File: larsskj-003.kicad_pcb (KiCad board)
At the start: 2 copper layers, 47.6 x 39 mm, 14 parts, among them J1 IDC connector, J2 Conn_02x01, J3 Conn_02x01, J4 Conn_02x01, J5 Conn_02x01, J6 Conn_02x01, J7 Conn_02x01, J8 Conn_02x01, J9 Conn_02x01

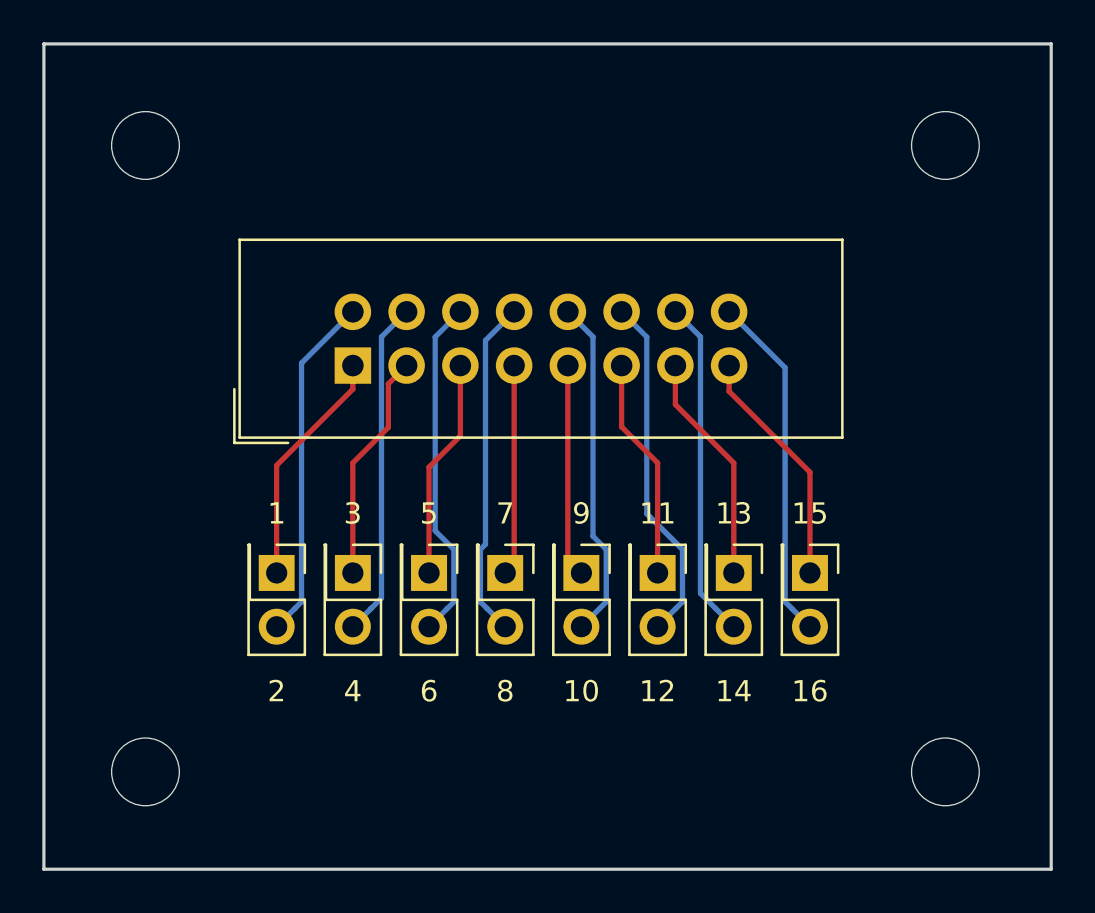
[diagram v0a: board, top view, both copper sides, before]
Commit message: Improved PCB layout
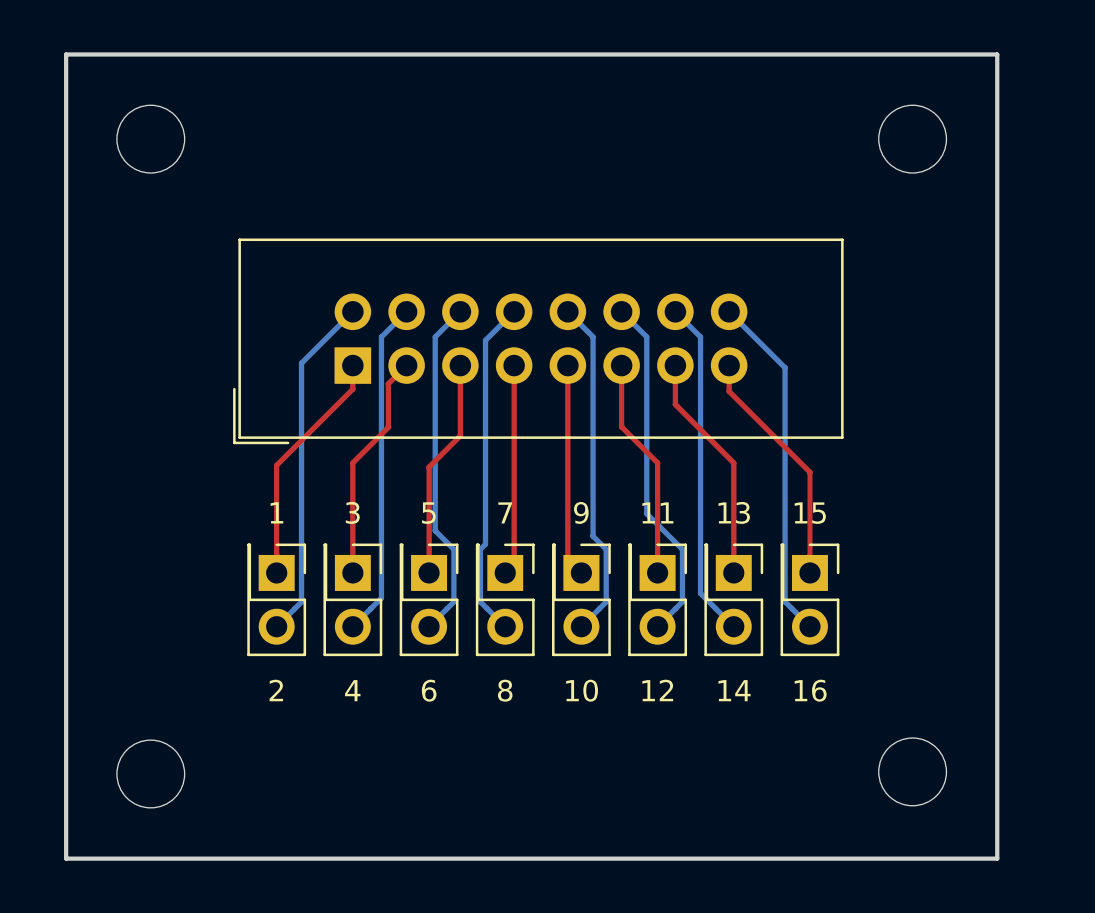
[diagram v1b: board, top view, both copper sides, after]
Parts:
- moved REF** 1.58 mm to (160.7, 80.3)
- moved REF** 1.55 mm to (160.7, 110.2)
- moved REF** 1.45 mm to (152.7, 95.8)
- moved REF** 0.39 mm to (124.7, 80.3)
- moved REF** 0.27 mm to (124.7, 110.3)
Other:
- board size 47.6 x 39 mm -> 44 x 38 mm
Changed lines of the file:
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@@
-(kicad_pcb (version 20171130) (host pcbnew "(5.0.1)-3")
+(kicad_pcb (version 20171130) (host pcbnew 5.0.2-bee76a0~70~ubuntu18.04.1)
   (general
     (thickness 1.6)
@@
     (solder_mask_min_width 0.25)
     (aux_axis_origin 0 0)
+    (grid_origin 120.65 114.3)
     (visible_elements 7FFFFFFF)
     (pcbplotparams
@@
   )
   (module MountingHole:MountingHole_3.2mm_M3 (layer F.Cu)
-    (at 162.2 110.2)
+    (at 160.65 110.2)
     (descr "Mounting Hole 3.2mm, no annular, M3")
     (tags "mounting hole 3.2mm no annular m3")
@@
   )
   (module MountingHole:MountingHole_3.2mm_M3 (layer F.Cu)
-    (at 124.4 110.2)
+    (at 124.65 110.3)
     (descr "Mounting Hole 3.2mm, no annular, M3")
     (tags "mounting hole 3.2mm no annular m3")
@@
   )
   (module MountingHole:MountingHole_3.2mm_M3 (layer F.Cu)
-    (at 162.2 80.6)
+    (at 160.65 80.3)
     (descr "Mounting Hole 3.2mm, no annular, M3")
     (tags "mounting hole 3.2mm no annular m3")
@@
   )
   (module Symbol:OSHW-Logo2_7.3x6mm_SilkScreen (layer B.Cu)
-    (at 151.2 95.8 180)
+    (at 152.65 95.8 180)
     (descr "Open Source Hardware Symbol")
     (tags "Logo Symbol OSHW")
     (attr virtual)
-    (fp_text reference REF** (at 0 0 180) (layer B.SilkS) hide
+    (fp_text reference REF** (at -9.45 -6.5 180) (layer B.SilkS) hide
       (effects (font (size 1 1) (thickness 0.15)) (justify mirror))
     )
@@
   )
   (module MountingHole:MountingHole_3.2mm_M3 (layer F.Cu)
-    (at 124.4 80.6)
+    (at 124.65 80.3)
     (descr "Mounting Hole 3.2mm, no annular, M3")
     (tags "mounting hole 3.2mm no annular m3")
@@
     (pad 1 np_thru_hole circle (at 0 0) (size 3.2 3.2) (drill 3.2) (layers *.Cu *.Mask))
   )
-  (gr_line (start 119.6 114.8) (end 119.6 75.8) (layer Edge.Cuts) (width 0.15))
-  (gr_line (start 167.2 114.8) (end 119.6 114.8) (layer Edge.Cuts) (width 0.15))
-  (gr_line (start 167.2 75.8) (end 167.2 114.8) (layer Edge.Cuts) (width 0.15))
-  (gr_line (start 119.6 75.8) (end 167.2 75.8) (layer Edge.Cuts) (width 0.15))
-  (gr_text larsskj-003-01 (at 138 97.4) (layer B.SilkS)
-    (effects (font (size 1 1) (thickness 0.2)) (justify mirror))
-  )
+  (gr_text larsskj-003-01 (at 139.65 95.3) (layer B.SilkS)
+    (effects (font (size 1.5 1.5) (thickness 0.3)) (justify mirror))
+  )
+  (gr_line (start 164.65 114.3) (end 120.65 114.3) (layer Edge.Cuts) (width 0.2))
+  (gr_line (start 164.65 76.3) (end 164.65 114.3) (layer Edge.Cuts) (width 0.2))
+  (gr_line (start 120.65 76.3) (end 164.65 76.3) (layer Edge.Cuts) (width 0.2))
+  (gr_line (start 120.65 114.3) (end 120.65 76.3) (layer Edge.Cuts) (width 0.2))
   (gr_text 16 (at 155.8 106.4) (layer F.SilkS)
     (effects (font (size 1 1) (thickness 0.2)))
@@
     (polygon
       (pts
-        (xy 119.6 75.8) (xy 167.2 75.8) (xy 167.2 114.8) (xy 119.6 114.8)
+        (xy 120.65 76.3) (xy 164.65 76.3) (xy 164.65 114.3) (xy 120.65 114.3)
       )
     )
@@
     (polygon
       (pts
-        (xy 119.6 75.8) (xy 167.2 75.8) (xy 167.2 114.8) (xy 119.6 114.8)
+        (xy 120.65 76.3) (xy 164.65 76.3) (xy 164.65 114.3) (xy 120.65 114.3)
       )
     )
